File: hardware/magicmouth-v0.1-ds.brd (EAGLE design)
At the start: 100 x 80 mm, 39 parts, among them IC1 LM386N, IC2 ATMEGA328P_PDIP, Q1 16Mhz, U1 ARDUINOR3-NOIOREF-NOTEXT

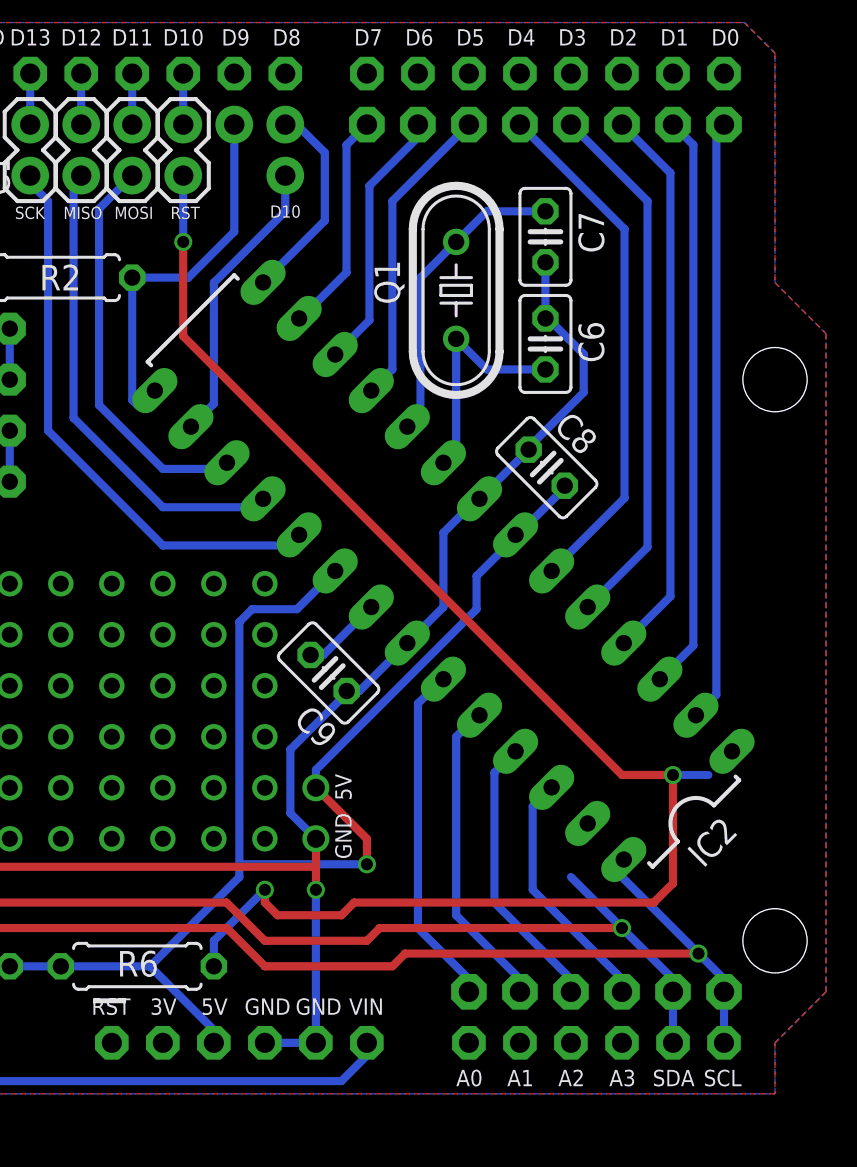
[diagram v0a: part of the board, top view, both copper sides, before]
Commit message: trace corrections
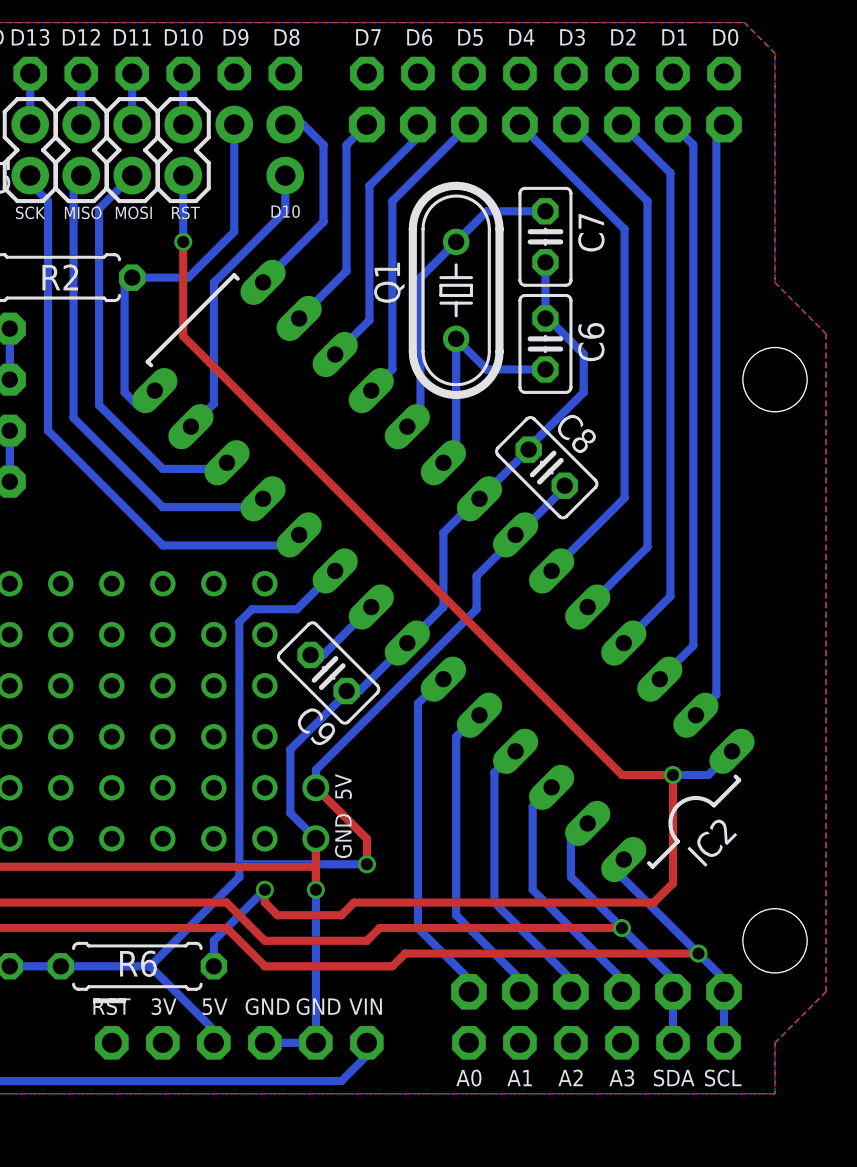
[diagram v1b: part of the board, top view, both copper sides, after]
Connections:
- net N$24 renamed D8
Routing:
- net SDA: track 70.3 -> 72.2 mm
- net SS: track 75.3 -> 77.0 mm
- net SIGNAL: track 18.0 -> 19.3 mm
- net MISO: track 23.1 -> 23.7 mm
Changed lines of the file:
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@@
 <setting verticaltext="up"/>
 </settings>
-<grid distance="1" unitdist="mil" unit="mil" style="lines" multiple="1" display="yes" altdistance="0.025" altunitdist="inch" altunit="inch"/>
+<grid distance="0.025" unitdist="inch" unit="inch" style="lines" multiple="1" display="yes" altdistance="0.025" altunitdist="inch" altunit="inch"/>
 <layers>
 <layer number="1" name="Top" color="4" fill="1" visible="yes" active="yes"/>
@@
 <contactref element="Q1" pad="2"/>
 <contactref element="C6" pad="2"/>
-<wire x1="60.325" y1="42.218153125" x2="60.325" y2="47.752" width="0.4064" layer="16"/>
 <wire x1="64.77" y1="46.228" x2="61.849" y2="46.228" width="0.4064" layer="16"/>
 <wire x1="61.849" y1="46.228" x2="60.325" y2="47.752" width="0.4064" layer="16"/>
 <contactref element="IC2" pad="9"/>
-<wire x1="59.69" y1="41.583153125" x2="60.325" y2="42.218153125" width="0.4064" layer="16"/>
+<wire x1="60.325" y1="47.752" x2="60.325" y2="42.218153125" width="0.4064" layer="16"/>
+<wire x1="60.325" y1="42.218153125" x2="59.69" y2="41.583153125" width="0.4064" layer="16"/>
 </signal>
 <signal name="N$11">
 <contactref element="Q1" pad="1"/>
 <contactref element="C7" pad="1"/>
-<wire x1="58.547" y1="44.03225625" x2="58.547" y2="50.8" width="0.4064" layer="16"/>
 <wire x1="58.547" y1="50.8" x2="60.325" y2="52.578" width="0.4064" layer="16"/>
 <wire x1="64.77" y1="54.102" x2="61.849" y2="54.102" width="0.4064" layer="16"/>
 <wire x1="61.849" y1="54.102" x2="60.325" y2="52.578" width="0.4064" layer="16"/>
 <contactref element="IC2" pad="10"/>
-<wire x1="57.893946875" y1="43.379203125" x2="58.547" y2="44.03225625" width="0.4064" layer="16"/>
+<wire x1="58.547" y1="50.8" x2="58.547" y2="44.03225625" width="0.4064" layer="16"/>
+<wire x1="58.547" y1="44.03225625" x2="57.893946875" y2="43.379203125" width="0.4064" layer="16"/>
 </signal>
 <signal name="SS">
@@
 <wire x1="48.26" y1="17.78" x2="50.8" y2="20.32" width="0.4064" layer="16"/>
 <contactref element="IC2" pad="1"/>
-<wire x1="72.878665625" y1="26.035" x2="74.058409375" y2="27.21474375" width="0" layer="19" extent="16-16"/>
+<wire x1="72.878665625" y1="26.035" x2="74.058409375" y2="27.21474375" width="0.4064" layer="16"/>
 </signal>
 <signal name="N$16">
@@
 <wire x1="56.007" y1="55.372" x2="56.007" y2="48.6764625" width="0.4064" layer="16"/>
 <contactref element="IC2" pad="12"/>
-<wire x1="54.30184375" y1="46.97130625" x2="56.007" y2="48.6764625" width="0.4064" layer="16"/>
+<wire x1="56.007" y1="48.6764625" x2="54.30184375" y2="46.97130625" width="0.4064" layer="16"/>
 </signal>
 <signal name="N$23">
 <contactref element="JP2" pad="8"/>
-<wire x1="52.705" y1="48.9665625" x2="52.7765625" y2="48.9665625" width="0.4064" layer="16"/>
-<wire x1="52.7765625" y1="48.9665625" x2="54.864" y2="51.054" width="0.4064" layer="16"/>
-<wire x1="54.864" y1="51.054" x2="54.864" y2="57.404" width="0.4064" layer="16"/>
 <wire x1="54.864" y1="57.404" x2="55.88" y2="58.42" width="0.4064" layer="16"/>
 <contactref element="IC2" pad="13"/>
-<wire x1="52.50579375" y1="48.76735625" x2="52.705" y2="48.9665625" width="0" layer="19" extent="16-16"/>
-</signal>
-<signal name="N$24">
-<contactref element="JP3" pad="1"/>
-<wire x1="51.816" y1="58.42" x2="52.3875" y2="58.42" width="0.4064" layer="16"/>
-<wire x1="52.3875" y1="58.42" x2="53.7845" y2="57.023" width="0.4064" layer="16"/>
-<wire x1="53.7845" y1="57.023" x2="53.7845" y2="53.638165625" width="0.4064" layer="16"/>
-<contactref element="IC2" pad="14"/>
-<wire x1="50.70974375" y1="50.563409375" x2="53.7845" y2="53.638165625" width="0.4064" layer="16"/>
+<wire x1="54.864" y1="57.404" x2="54.864" y2="51.1255625" width="0.4064" layer="16"/>
+<wire x1="54.864" y1="51.1255625" x2="52.50579375" y2="48.76735625" width="0.4064" layer="16"/>
 </signal>
 <signal name="SIGNAL">
 <contactref element="R2" pad="1"/>
+<wire x1="49.276" y1="53.086" x2="46.99" y2="50.8" width="0.4064" layer="16"/>
+<wire x1="46.99" y1="50.8" x2="44.196" y2="50.8" width="0.4064" layer="16"/>
+<wire x1="44.45" y1="44.45" x2="44.596334375" y2="44.45" width="0.4064" layer="16"/>
+<contactref element="IC2" pad="15"/>
 <contactref element="JP3" pad="2"/>
 <wire x1="49.276" y1="58.42" x2="49.276" y2="53.086" width="0.4064" layer="16"/>
-<wire x1="49.276" y1="53.086" x2="46.99" y2="50.8" width="0.4064" layer="16"/>
-<wire x1="46.99" y1="50.8" x2="44.196" y2="50.8" width="0.4064" layer="16"/>
-<wire x1="44.196" y1="50.8" x2="44.196" y2="44.704" width="0.4064" layer="16"/>
-<wire x1="44.196" y1="44.704" x2="44.45" y2="44.45" width="0.4064" layer="16"/>
-<wire x1="44.45" y1="44.45" x2="44.596334375" y2="44.45" width="0.4064" layer="16"/>
-<contactref element="IC2" pad="15"/>
-<wire x1="45.3215875" y1="45.175253125" x2="44.596334375" y2="44.45" width="0" layer="19" extent="16-16"/>
+<wire x1="44.596334375" y1="44.45" x2="45.3215875" y2="45.175253125" width="0.4064" layer="16"/>
+<wire x1="44.45" y1="44.45" x2="43.815" y2="45.085" width="0.4064" layer="16"/>
+<wire x1="43.815" y1="45.085" x2="43.815" y2="50.419" width="0.4064" layer="16"/>
+<wire x1="43.815" y1="50.419" x2="44.196" y2="50.8" width="0.4064" layer="16"/>
 </signal>
 <signal name="MISO">
 <wire x1="41.275" y1="43.815" x2="45.72" y2="39.37" width="0.4064" layer="16"/>
-<wire x1="45.72" y1="39.37" x2="50.29264375" y2="39.37" width="0.4064" layer="16"/>
 <contactref element="JP6" pad="2"/>
 <wire x1="41.275" y1="43.815" x2="41.275" y2="55.499" width="0.4064" layer="16"/>
 <wire x1="41.275" y1="55.499" x2="41.656" y2="55.88" width="0.4064" layer="16"/>
 <contactref element="IC2" pad="18"/>
-<wire x1="50.29264375" y1="39.37" x2="50.70974375" y2="39.7871" width="0" layer="19" extent="16-16"/>
+<wire x1="45.72" y1="39.37" x2="50.29264375" y2="39.37" width="0.4064" layer="16"/>
+<wire x1="50.29264375" y1="39.37" x2="50.70974375" y2="39.7871" width="0.4064" layer="16"/>
 </signal>
 <signal name="SCK">
 <contactref element="JP5" pad="2"/>
-<contactref element="IC2" pad="19"/>
 <wire x1="39.116" y1="55.88" x2="39.116" y2="55.499" width="0.4064" layer="16"/>
 <wire x1="39.116" y1="55.499" x2="40.005" y2="54.61" width="0.4064" layer="16"/>
 <wire x1="40.005" y1="54.61" x2="40.005" y2="43.18" width="0.4064" layer="16"/>
 <wire x1="40.005" y1="43.18" x2="45.72" y2="37.465" width="0.4064" layer="16"/>
+<contactref element="IC2" pad="19"/>
 <wire x1="45.72" y1="37.465" x2="51.97974375" y2="37.465" width="0.4064" layer="16"/>
 <wire x1="51.97974375" y1="37.465" x2="52.50579375" y2="37.99105" width="0.4064" layer="16"/>
@@
 <signal name="MOSI">
 <wire x1="45.72" y1="41.275" x2="42.545" y2="44.45" width="0.4064" layer="16"/>
-<wire x1="45.72" y1="41.275" x2="48.6055375" y2="41.275" width="0.4064" layer="16"/>
 <contactref element="JP7" pad="2"/>
 <wire x1="42.545" y1="44.45" x2="42.545" y2="54.229" width="0.4064" layer="16"/>
 <wire x1="42.545" y1="54.229" x2="44.196" y2="55.88" width="0.4064" layer="16"/>
 <contactref element="IC2" pad="17"/>
-<wire x1="48.6055375" y1="41.275" x2="48.913690625" y2="41.583153125" width="0" layer="19" extent="16-16"/>
+<wire x1="45.72" y1="41.275" x2="48.6055375" y2="41.275" width="0.4064" layer="16"/>
+<wire x1="48.6055375" y1="41.275" x2="48.913690625" y2="41.583153125" width="0.4064" layer="16"/>
 </signal>
 <signal name="+3V3">
@@
 <wire x1="51.816" y1="55.88" x2="51.816" y2="54.102" width="0.4064" layer="16"/>
 <wire x1="51.816" y1="54.102" x2="48.26" y2="50.546" width="0.4064" layer="16"/>
+<contactref element="IC2" pad="16"/>
 <wire x1="48.26" y1="50.546" x2="48.26" y2="44.5215625" width="0.4064" layer="16"/>
-<contactref element="IC2" pad="16"/>
-<wire x1="47.117640625" y1="43.379203125" x2="48.26" y2="44.5215625" width="0.4064" layer="16"/>
+<wire x1="48.26" y1="44.5215625" x2="47.117640625" y2="43.379203125" width="0.4064" layer="16"/>
 </signal>
 <signal name="N$87">
@@
 <wire x1="71.12" y1="15.875" x2="68.58" y2="18.415" width="0.4064" layer="16"/>
 <wire x1="68.58" y1="18.415" x2="66.04" y2="20.955" width="0.4064" layer="16"/>
-<wire x1="66.04" y1="20.955" x2="66.04" y2="22.86" width="0" layer="19" extent="1-16"/>
 <contactref element="U1" pad="A4"/>
-<wire x1="71.12" y1="15.24" x2="71.12" y2="12.7" width="0.4064" layer="16"/>
 <contactref element="JP10" pad="5"/>
 <wire x1="12.7" y1="15.24" x2="13.335" y2="15.24" width="0.4064" layer="16"/>
@@
 <wire x1="66.874203125" y1="23.622640625" x2="66.802640625" y2="23.622640625" width="0.4064" layer="16"/>
 <wire x1="66.802640625" y1="23.622640625" x2="66.04" y2="22.86" width="0.4064" layer="16"/>
+<wire x1="66.04" y1="20.955" x2="66.04" y2="22.86" width="0.4064" layer="16"/>
+<wire x1="71.12" y1="12.7" x2="71.12" y2="15.24" width="0.4064" layer="16"/>
 </signal>
 <signal name="SCL">
 <contactref element="JP4" pad="6"/>
 <contactref element="U1" pad="A5"/>
-<wire x1="73.66" y1="15.24" x2="73.66" y2="12.7" width="0.4064" layer="16"/>
 <wire x1="73.66" y1="15.24" x2="73.66" y2="15.875" width="0.4064" layer="16"/>
 <wire x1="73.66" y1="15.875" x2="72.39" y2="17.145" width="0.4064" layer="16"/>
@@
 <wire x1="68.670253125" y1="21.8265875" x2="68.670253125" y2="21.680253125" width="0.4064" layer="16"/>
 <wire x1="68.670253125" y1="21.680253125" x2="68.58" y2="21.59" width="0.4064" layer="16"/>
+<wire x1="73.66" y1="12.7" x2="73.66" y2="15.24" width="0.4064" layer="16"/>
 </signal>
 <signal name="N$3">
@@
 <wire x1="53.711975" y1="32.013025" x2="56.097896875" y2="34.398946875" width="0.4064" layer="16"/>
 </signal>
+<signal name="D8">
+<contactref element="IC2" pad="14"/>
+<contactref element="JP3" pad="1"/>
+<wire x1="51.816" y1="58.42" x2="52.705" y2="58.42" width="0.4064" layer="16"/>
+<wire x1="52.705" y1="58.42" x2="53.721" y2="57.404" width="0.4064" layer="16"/>
+<wire x1="53.721" y1="57.404" x2="53.721" y2="53.574665625" width="0.4064" layer="16"/>
+<wire x1="53.721" y1="53.574665625" x2="50.70974375" y2="50.563409375" width="0.4064" layer="16"/>
+</signal>
 </signals>
